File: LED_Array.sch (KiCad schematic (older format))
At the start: 64 parts

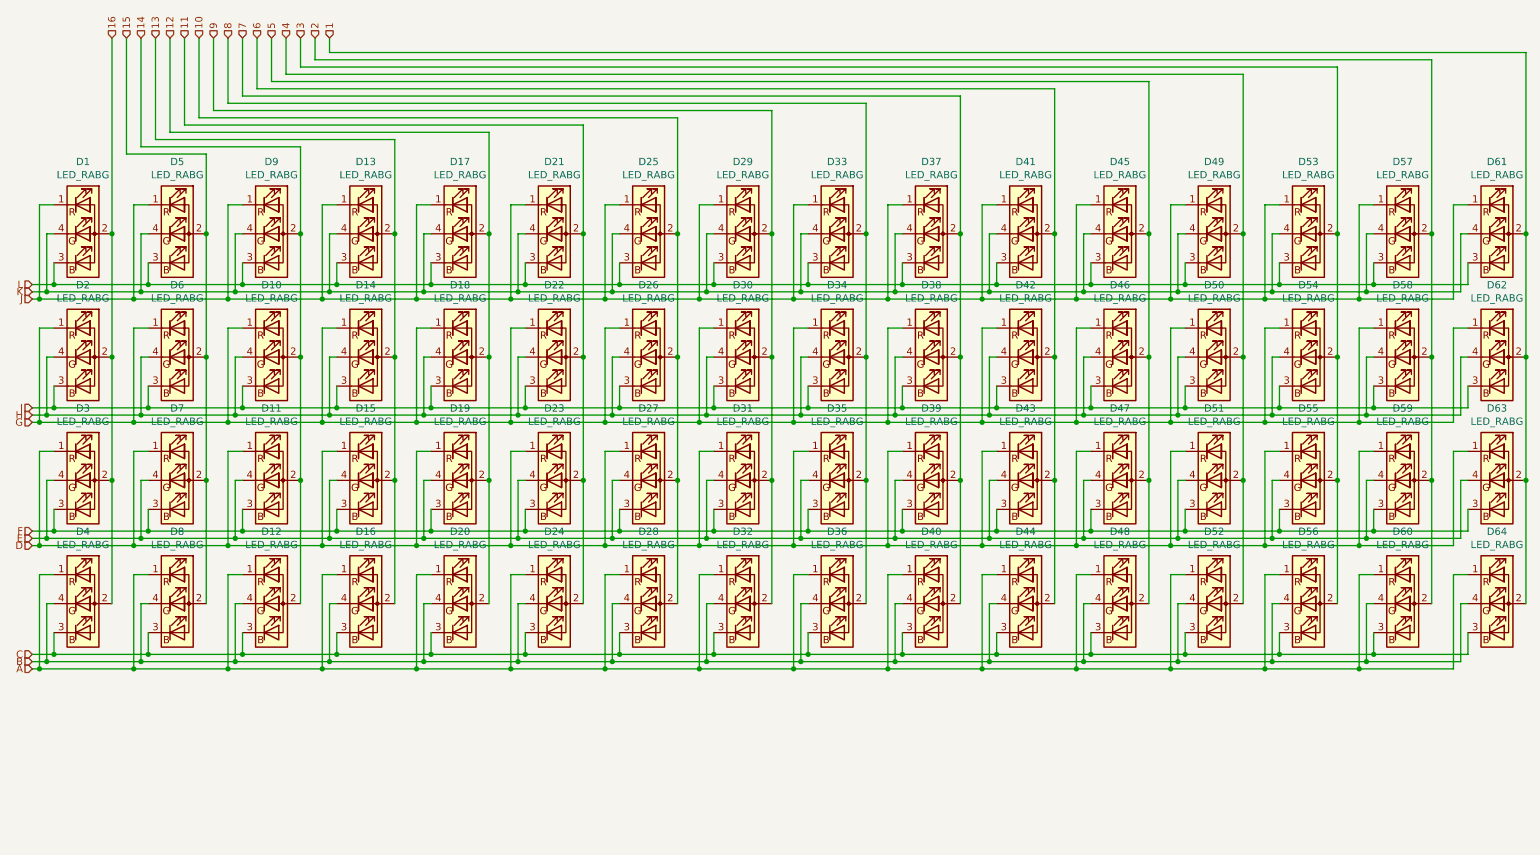
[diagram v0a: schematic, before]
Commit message: monocolor? or it could actually go multicolor?
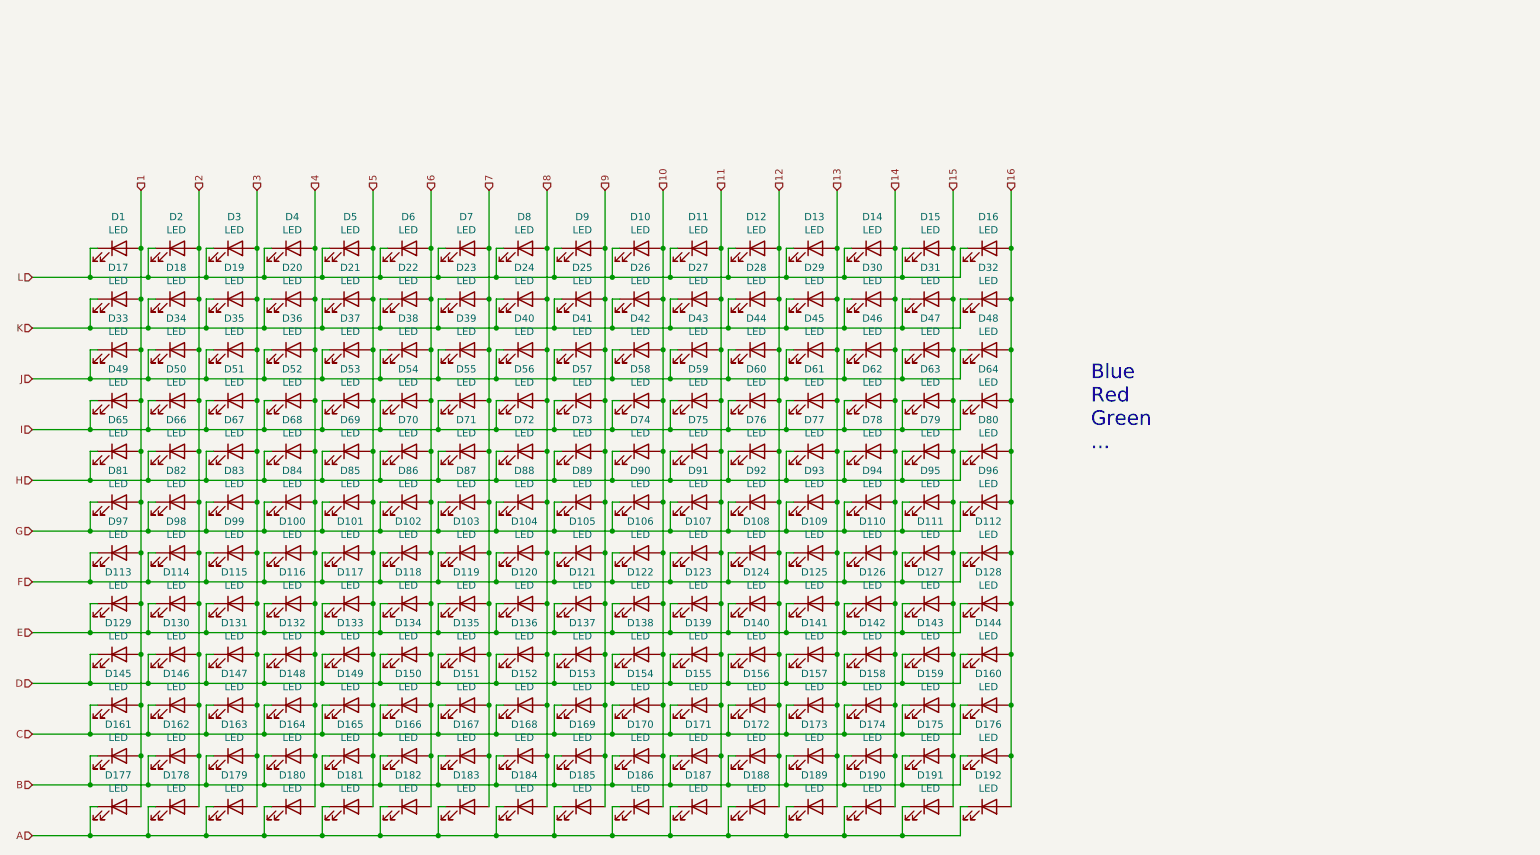
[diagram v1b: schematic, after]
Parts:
- removed D1, D10, D11, D12, D13, D14, D15, D16, D17, D18, D19, D2, D20, D21, D22, D23, D24, D25, D26, D27, D28, D29, D3, D30, D31, D32, D33, D34, D35, D36, D37, D38, D39, D4, D40, D41, D42, D43, D44, D45, D46, D47, D48, D49, D5, D50, D51, D52, D53, D54, D55, D56, D57, D58, D59, D6, D60, D61, D62, D63, D64, D7, D8, D9: LED_RABG, KiCad:RGB_LED_1206_reverse, symbol Device:LED_RABG
- added D1, D10, D100, D101, D102, D103, D104, D105, D106, D107, D108, D109, D11, D110, D111, D112, D113, D114, D115, D116, D117, D118, D119, D12, D120, D121, D122, D123, D124, D125, D126, D127, D128, D129, D13, D130, D131, D132, D133, D134, D135, D136, D137, D138, D139, D14, D140, D141, D142, D143, D144, D145, D146, D147, D148, D149, D15, D150, D151, D152, D153, D154, D155, D156, D157, D158, D159, D16, D160, D161, D162, D163, D164, D165, D166, D167, D168, D169, D17, D170, D171, D172, D173, D174, D175, D176, D177, D178, D179, D18, D180, D181, D182, D183, D184, D185, D186, D187, D188, D189, D19, D190, D191, D192, D2, D20, D21, D22, D23, D24, D25, D26, D27, D28, D29, D3, D30, D31, D32, D33, D34, D35, D36, D37, D38, D39, D4, D40, D41, D42, D43, D44, D45, D46, D47, D48, D49, D5, D50, D51, D52, D53, D54, D55, D56, D57, D58, D59, D6, D60, D61, D62, D63, D64, D65, D66, D67, D68, D69, D7, D70, D71, D72, D73, D74, D75, D76, D77, D78, D79, D8, D80, D81, D82, D83, D84, D85, D86, D87, D88, D89, D9, D90, D91, D92, D93, D94, D95, D96, D97, D98, D99: LED, KiCad:LED_0603_1608Metric_HideText, symbol Device:LED
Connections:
- net 1: now also D1.2 (A), D113.2 (A), D129.2 (A), D145.2 (A), D161.2 (A), D17.2 (A), D177.2 (A), D33.2 (A), D49.2 (A), D65.2 (A), D81.2 (A), D97.2 (A)
- net 10: now also D10.2 (A), D106.2 (A), D122.2 (A), D138.2 (A), D154.2 (A), D170.2 (A), D186.2 (A), D26.2 (A), D42.2 (A), D58.2 (A), D74.2 (A), D90.2 (A)
- net 11: now also D107.2 (A), D11.2 (A), D123.2 (A), D139.2 (A), D155.2 (A), D171.2 (A), D187.2 (A), D27.2 (A), D43.2 (A), D59.2 (A), D75.2 (A), D91.2 (A)
- net 12: now also D108.2 (A), D12.2 (A), D124.2 (A), D140.2 (A), D156.2 (A), D172.2 (A), D188.2 (A), D28.2 (A), D44.2 (A), D60.2 (A), D76.2 (A), D92.2 (A)
- net 13: now also D109.2 (A), D125.2 (A), D13.2 (A), D141.2 (A), D157.2 (A), D173.2 (A), D189.2 (A), D29.2 (A), D45.2 (A), D61.2 (A), D77.2 (A), D93.2 (A)
- net 14: now also D110.2 (A), D126.2 (A), D14.2 (A), D142.2 (A), D158.2 (A), D174.2 (A), D190.2 (A), D30.2 (A), D46.2 (A), D62.2 (A), D78.2 (A), D94.2 (A)
- net 15: now also D111.2 (A), D127.2 (A), D143.2 (A), D15.2 (A), D159.2 (A), D175.2 (A), D191.2 (A), D31.2 (A), D47.2 (A), D63.2 (A), D79.2 (A), D95.2 (A)
- net 16: now also D112.2 (A), D128.2 (A), D144.2 (A), D16.2 (A), D160.2 (A), D176.2 (A), D192.2 (A), D32.2 (A), D48.2 (A), D64.2 (A), D80.2 (A), D96.2 (A)
- net 2: now also D114.2 (A), D130.2 (A), D146.2 (A), D162.2 (A), D178.2 (A), D18.2 (A), D2.2 (A), D34.2 (A), D50.2 (A), D66.2 (A), D82.2 (A), D98.2 (A)
- net 3: now also D115.2 (A), D131.2 (A), D147.2 (A), D163.2 (A), D179.2 (A), D19.2 (A), D3.2 (A), D35.2 (A), D51.2 (A), D67.2 (A), D83.2 (A), D99.2 (A)
- net 4: now also D100.2 (A), D116.2 (A), D132.2 (A), D148.2 (A), D164.2 (A), D180.2 (A), D20.2 (A), D36.2 (A), D4.2 (A), D52.2 (A), D68.2 (A), D84.2 (A)
- net 5: now also D101.2 (A), D117.2 (A), D133.2 (A), D149.2 (A), D165.2 (A), D181.2 (A), D21.2 (A), D37.2 (A), D5.2 (A), D53.2 (A), D69.2 (A), D85.2 (A)
- net 6: now also D102.2 (A), D118.2 (A), D134.2 (A), D150.2 (A), D166.2 (A), D182.2 (A), D22.2 (A), D38.2 (A), D54.2 (A), D6.2 (A), D70.2 (A), D86.2 (A)
- net 7: now also D103.2 (A), D119.2 (A), D135.2 (A), D151.2 (A), D167.2 (A), D183.2 (A), D23.2 (A), D39.2 (A), D55.2 (A), D7.2 (A), D71.2 (A), D87.2 (A)
- net 8: now also D104.2 (A), D120.2 (A), D136.2 (A), D152.2 (A), D168.2 (A), D184.2 (A), D24.2 (A), D40.2 (A), D56.2 (A), D72.2 (A), D8.2 (A), D88.2 (A)
- net 9: now also D105.2 (A), D121.2 (A), D137.2 (A), D153.2 (A), D169.2 (A), D185.2 (A), D25.2 (A), D41.2 (A), D57.2 (A), D73.2 (A), D89.2 (A), D9.2 (A)
- net A: now also D177.1 (K), D178.1 (K), D179.1 (K), D180.1 (K), D181.1 (K), D182.1 (K), D183.1 (K), D184.1 (K), D185.1 (K), D186.1 (K), D187.1 (K), D188.1 (K), D189.1 (K), D190.1 (K), D191.1 (K), D192.1 (K)
- net B: now also D161.1 (K), D162.1 (K), D163.1 (K), D164.1 (K), D165.1 (K), D166.1 (K), D167.1 (K), D168.1 (K), D169.1 (K), D170.1 (K), D171.1 (K), D172.1 (K), D173.1 (K), D174.1 (K), D175.1 (K), D176.1 (K)
- net C: now also D145.1 (K), D146.1 (K), D147.1 (K), D148.1 (K), D149.1 (K), D150.1 (K), D151.1 (K), D152.1 (K), D153.1 (K), D154.1 (K), D155.1 (K), D156.1 (K), D157.1 (K), D158.1 (K), D159.1 (K), D160.1 (K)
- net D: now also D129.1 (K), D130.1 (K), D131.1 (K), D132.1 (K), D133.1 (K), D134.1 (K), D135.1 (K), D136.1 (K), D137.1 (K), D138.1 (K), D139.1 (K), D140.1 (K), D141.1 (K), D142.1 (K), D143.1 (K), D144.1 (K)
- net E: now also D113.1 (K), D114.1 (K), D115.1 (K), D116.1 (K), D117.1 (K), D118.1 (K), D119.1 (K), D120.1 (K), D121.1 (K), D122.1 (K), D123.1 (K), D124.1 (K), D125.1 (K), D126.1 (K), D127.1 (K), D128.1 (K)
- net F: now also D100.1 (K), D101.1 (K), D102.1 (K), D103.1 (K), D104.1 (K), D105.1 (K), D106.1 (K), D107.1 (K), D108.1 (K), D109.1 (K), D110.1 (K), D111.1 (K), D112.1 (K), D97.1 (K), D98.1 (K), D99.1 (K)
- net G: now also D81.1 (K), D82.1 (K), D83.1 (K), D84.1 (K), D85.1 (K), D86.1 (K), D87.1 (K), D88.1 (K), D89.1 (K), D90.1 (K), D91.1 (K), D92.1 (K), D93.1 (K), D94.1 (K), D95.1 (K), D96.1 (K)
- net H: now also D65.1 (K), D66.1 (K), D67.1 (K), D68.1 (K), D69.1 (K), D70.1 (K), D71.1 (K), D72.1 (K), D73.1 (K), D74.1 (K), D75.1 (K), D76.1 (K), D77.1 (K), D78.1 (K), D79.1 (K), D80.1 (K)
- net I: now also D49.1 (K), D50.1 (K), D51.1 (K), D52.1 (K), D53.1 (K), D54.1 (K), D55.1 (K), D56.1 (K), D57.1 (K), D58.1 (K), D59.1 (K), D60.1 (K), D61.1 (K), D62.1 (K), D63.1 (K), D64.1 (K)
- net J: now also D33.1 (K), D34.1 (K), D35.1 (K), D36.1 (K), D37.1 (K), D38.1 (K), D39.1 (K), D40.1 (K), D41.1 (K), D42.1 (K), D43.1 (K), D44.1 (K), D45.1 (K), D46.1 (K), D47.1 (K), D48.1 (K)
- net K: now also D17.1 (K), D18.1 (K), D19.1 (K), D20.1 (K), D21.1 (K), D22.1 (K), D23.1 (K), D24.1 (K), D25.1 (K), D26.1 (K), D27.1 (K), D28.1 (K), D29.1 (K), D30.1 (K), D31.1 (K), D32.1 (K)
- net L: now also D1.1 (K), D10.1 (K), D11.1 (K), D12.1 (K), D13.1 (K), D14.1 (K), D15.1 (K), D16.1 (K), D2.1 (K), D3.1 (K), D4.1 (K), D5.1 (K), D6.1 (K), D7.1 (K), D8.1 (K), D9.1 (K)
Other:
- note added: "Blue\nRed\nGreen\n..."
